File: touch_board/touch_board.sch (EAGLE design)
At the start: 43 parts, among them IC1 PIC18F47K42-I_PT, IC2 MAX203EEWP, K1 G6K-2P, X1 RS-232-1, X2 RS-232-2, X3 POWER, X4 GLORY, X5 Relay conn

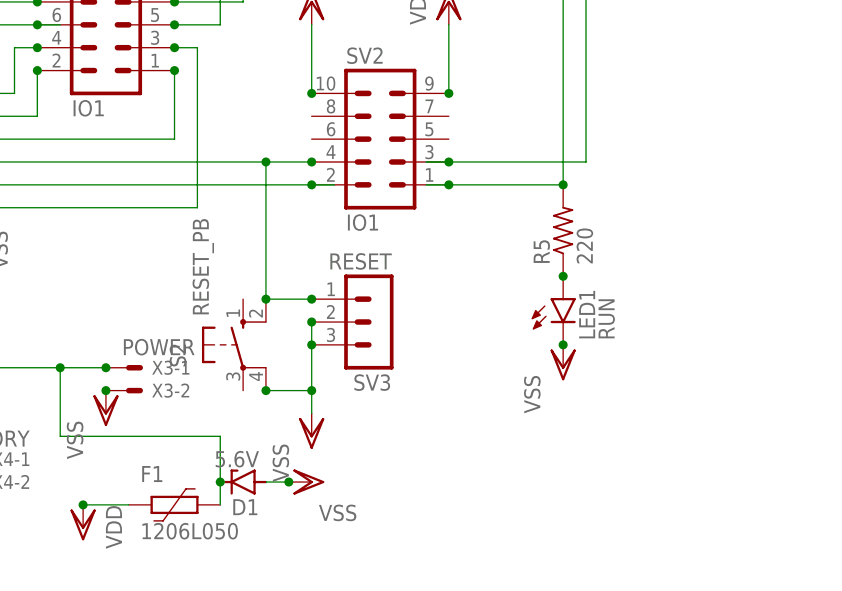
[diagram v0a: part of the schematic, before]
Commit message: updatei# Please enter the commit message for your changes. Lines starting
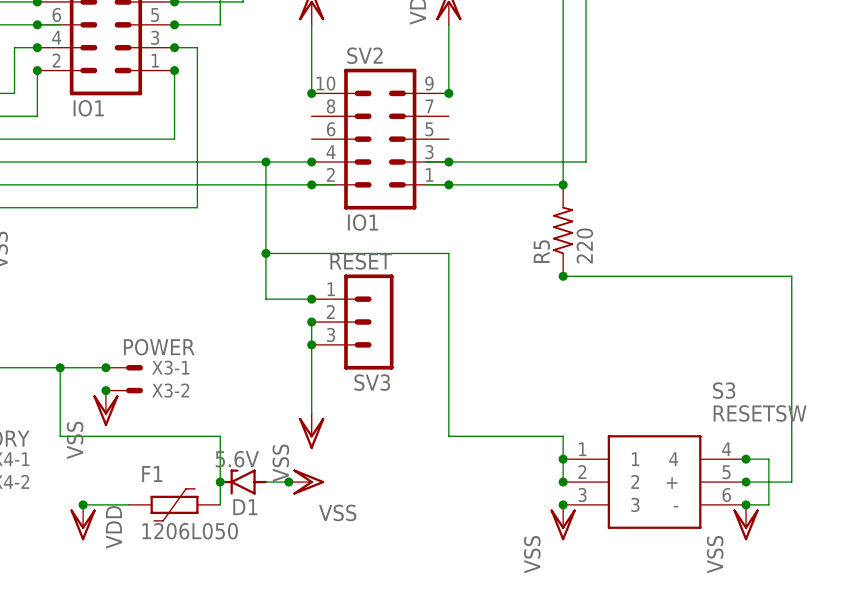
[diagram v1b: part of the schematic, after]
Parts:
- removed LED1: RUN, led:LEDCHIPLED_1206
- removed S2: RESET_PB, switch-omron:10-XX
- added S3: RESETSW, SamacSys_Parts:B3W-9000-Y1N
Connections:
- net N$2: now also S3.1, S3.2; no longer S2.S1
- net N$9: now also S3.+; no longer LED1.A
- net VSS: now also S3.-, S3.3, S3.4; no longer LED1.C, S2.P1
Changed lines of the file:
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@@
 <part name="VSS9" library="supply1" library_urn="urn:adsk.eagle:library:371" deviceset="VSS" device=""/>
 <part name="R5" library="rcl" library_urn="urn:adsk.eagle:library:334" deviceset="R-US_" device="R0805" package3d_urn="urn:adsk.eagle:package:23553/2" value="220"/>
-<part name="LED1" library="led" library_urn="urn:adsk.eagle:library:259" deviceset="LED" device="CHIPLED_1206" package3d_urn="urn:adsk.eagle:package:15823/2" value="RUN"/>
-<part name="VSS10" library="supply1" library_urn="urn:adsk.eagle:library:371" deviceset="VSS" device=""/>
 <part name="LED2" library="led" library_urn="urn:adsk.eagle:library:259" deviceset="LED" device="CHIPLED_1206" package3d_urn="urn:adsk.eagle:package:15823/2" value="MODE"/>
 <part name="VSS11" library="supply1" library_urn="urn:adsk.eagle:library:371" deviceset="VSS" device=""/>
@@
 <part name="VSS19" library="supply1" library_urn="urn:adsk.eagle:library:371" deviceset="VSS" device=""/>
 <part name="VDD12" library="supply1" library_urn="urn:adsk.eagle:library:371" deviceset="VDD" device=""/>
-<part name="S2" library="switch-omron" library_urn="urn:adsk.eagle:library:377" deviceset="10-XX" device="" package3d_urn="urn:adsk.eagle:package:27496/1" value="RESET_PB"/>
 <part name="X4" library="con-molex" library_urn="urn:adsk.eagle:library:165" deviceset="22-23-2021" device="" package3d_urn="urn:adsk.eagle:package:8078633/1" value="GLORY"/>
 <part name="VSS20" library="supply1" library_urn="urn:adsk.eagle:library:371" deviceset="VSS" device=""/>
@@
 <part name="D1" library="diode" library_urn="urn:adsk.eagle:library:210" deviceset="ZENER-DIODE" device="ZD-7.5" package3d_urn="urn:adsk.eagle:package:43411/1" value="5.6V"/>
 <part name="VSS23" library="supply1" library_urn="urn:adsk.eagle:library:371" deviceset="VSS" device=""/>
+<part name="S3" library="SamacSys_Parts" deviceset="B3W-9000-Y1N" device="" value="RESETSW"/>
+<part name="VSS24" library="supply1" library_urn="urn:adsk.eagle:library:371" deviceset="VSS" device=""/>
+<part name="VSS25" library="supply1" library_urn="urn:adsk.eagle:library:371" deviceset="VSS" device=""/>
 </parts>
 <sheets>
@@
 <attribute name="VALUE" x="168.402" y="-31.75" size="1.778" layer="96" rot="R90"/>
 </instance>
-<instance part="LED1" gate="G$1" x="165.1" y="-35.56" smashed="yes">
-<attribute name="NAME" x="168.656" y="-40.132" size="1.778" layer="95" rot="R90"/>
-<attribute name="VALUE" x="170.815" y="-40.132" size="1.778" layer="96" rot="R90"/>
-</instance>
-<instance part="VSS10" gate="G$1" x="165.1" y="-43.18" smashed="yes">
-<attribute name="VALUE" x="162.56" y="-48.26" size="1.778" layer="96" rot="R90"/>
-</instance>
 <instance part="LED2" gate="G$1" x="78.74" y="86.36" smashed="yes">
 <attribute name="NAME" x="82.296" y="81.788" size="1.778" layer="95" rot="R90"/>
@@
 <attribute name="VALUE" x="43.18" y="15.24" size="1.778" layer="96" rot="R90"/>
 </instance>
-<instance part="S2" gate="1" x="129.54" y="-40.64" smashed="yes">
-<attribute name="NAME" x="123.19" y="-43.18" size="1.778" layer="95" rot="R90"/>
-<attribute name="VALUE" x="125.73" y="-37.465" size="1.778" layer="96" rot="R90"/>
-</instance>
 <instance part="X4" gate="-1" x="99.06" y="-53.34" smashed="yes">
 <attribute name="NAME" x="101.6" y="-54.102" size="1.524" layer="95"/>
@@
 <instance part="VSS23" gate="G$1" x="137.16" y="-55.88" smashed="yes" rot="R90">
 <attribute name="VALUE" x="142.24" y="-58.42" size="1.778" layer="96" rot="R180"/>
+</instance>
+<instance part="S3" gate="G$1" x="165.1" y="-53.34" smashed="yes">
+<attribute name="NAME" x="181.61" y="-45.72" size="1.778" layer="95" align="center-left"/>
+<attribute name="VALUE" x="181.61" y="-48.26" size="1.778" layer="96" align="center-left"/>
+</instance>
+<instance part="VSS24" gate="G$1" x="165.1" y="-60.96" smashed="yes">
+<attribute name="VALUE" x="162.56" y="-66.04" size="1.778" layer="96" rot="R90"/>
+</instance>
+<instance part="VSS25" gate="G$1" x="185.42" y="-60.96" smashed="yes">
+<attribute name="VALUE" x="182.88" y="-66.04" size="1.778" layer="96" rot="R90"/>
 </instance>
 </instances>
@@
 </segment>
 <segment>
-<pinref part="LED1" gate="G$1" pin="C"/>
-<pinref part="VSS10" gate="G$1" pin="VSS"/>
-<junction x="165.1" y="-40.64"/>
-</segment>
-<segment>
 <pinref part="LED2" gate="G$1" pin="C"/>
 <pinref part="VSS11" gate="G$1" pin="VSS"/>
@@
 <pinref part="SV3" gate="G$1" pin="3"/>
 <junction x="137.16" y="-40.64"/>
-<wire x1="137.16" y1="-40.64" x2="137.16" y2="-45.72" width="0.1524" layer="91"/>
+<wire x1="137.16" y1="-40.64" x2="137.16" y2="-48.26" width="0.1524" layer="91"/>
 <junction x="137.16" y="-38.1"/>
-<pinref part="S2" gate="1" pin="P1"/>
-<wire x1="137.16" y1="-45.72" x2="137.16" y2="-48.26" width="0.1524" layer="91"/>
-<wire x1="132.08" y1="-45.72" x2="137.16" y2="-45.72" width="0.1524" layer="91"/>
-<junction x="132.08" y="-45.72"/>
-<junction x="137.16" y="-45.72"/>
 </segment>
 <segment>
@@
 <wire x1="134.62" y1="-55.88" x2="132.08" y2="-55.88" width="0.1524" layer="91"/>
 <junction x="134.62" y="-55.88"/>
+</segment>
+<segment>
+<pinref part="S3" gate="G$1" pin="3"/>
+<pinref part="VSS24" gate="G$1" pin="VSS"/>
+<junction x="165.1" y="-58.42"/>
+</segment>
+<segment>
+<pinref part="S3" gate="G$1" pin="-"/>
+<pinref part="VSS25" gate="G$1" pin="VSS"/>
+<junction x="185.42" y="-58.42"/>
+<pinref part="S3" gate="G$1" pin="4"/>
+<wire x1="185.42" y1="-53.34" x2="187.96" y2="-53.34" width="0.1524" layer="91"/>
+<wire x1="187.96" y1="-53.34" x2="187.96" y2="-58.42" width="0.1524" layer="91"/>
+<wire x1="187.96" y1="-58.42" x2="185.42" y2="-58.42" width="0.1524" layer="91"/>
+<junction x="185.42" y="-53.34"/>
 </segment>
 </net>
@@
 <junction x="137.16" y="-20.32"/>
 <wire x1="132.08" y1="-20.32" x2="137.16" y2="-20.32" width="0.1524" layer="91"/>
-<wire x1="132.08" y1="-20.32" x2="132.08" y2="-35.56" width="0.1524" layer="91"/>
+<wire x1="132.08" y1="-20.32" x2="132.08" y2="-30.48" width="0.1524" layer="91"/>
 <pinref part="SV3" gate="G$1" pin="1"/>
+<wire x1="132.08" y1="-30.48" x2="132.08" y2="-35.56" width="0.1524" layer="91"/>
 <wire x1="132.08" y1="-35.56" x2="137.16" y2="-35.56" width="0.1524" layer="91"/>
 <junction x="137.16" y="-35.56"/>
 <junction x="132.08" y="-20.32"/>
-<pinref part="S2" gate="1" pin="S1"/>
-<junction x="132.08" y="-35.56"/>
+<pinref part="S3" gate="G$1" pin="2"/>
+<pinref part="S3" gate="G$1" pin="1"/>
+<wire x1="165.1" y1="-55.88" x2="165.1" y2="-53.34" width="0.1524" layer="91"/>
+<wire x1="165.1" y1="-53.34" x2="165.1" y2="-50.8" width="0.1524" layer="91"/>
+<wire x1="165.1" y1="-50.8" x2="152.4" y2="-50.8" width="0.1524" layer="91"/>
+<wire x1="152.4" y1="-50.8" x2="152.4" y2="-30.48" width="0.1524" layer="91"/>
+<wire x1="152.4" y1="-30.48" x2="132.08" y2="-30.48" width="0.1524" layer="91"/>
+<junction x="132.08" y="-30.48"/>
+<junction x="165.1" y="-53.34"/>
+<junction x="165.1" y="-55.88"/>
 </segment>
 </net>
@@
 <segment>
 <pinref part="R5" gate="G$1" pin="1"/>
-<pinref part="LED1" gate="G$1" pin="A"/>
+<wire x1="165.1" y1="-33.02" x2="190.5" y2="-33.02" width="0.1524" layer="91"/>
+<wire x1="190.5" y1="-33.02" x2="190.5" y2="-55.88" width="0.1524" layer="91"/>
+<pinref part="S3" gate="G$1" pin="+"/>
+<wire x1="190.5" y1="-55.88" x2="185.42" y2="-55.88" width="0.1524" layer="91"/>
+<junction x="185.42" y="-55.88"/>
 <junction x="165.1" y="-33.02"/>
 </segment>
